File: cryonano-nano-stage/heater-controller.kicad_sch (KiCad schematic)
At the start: 0 parts

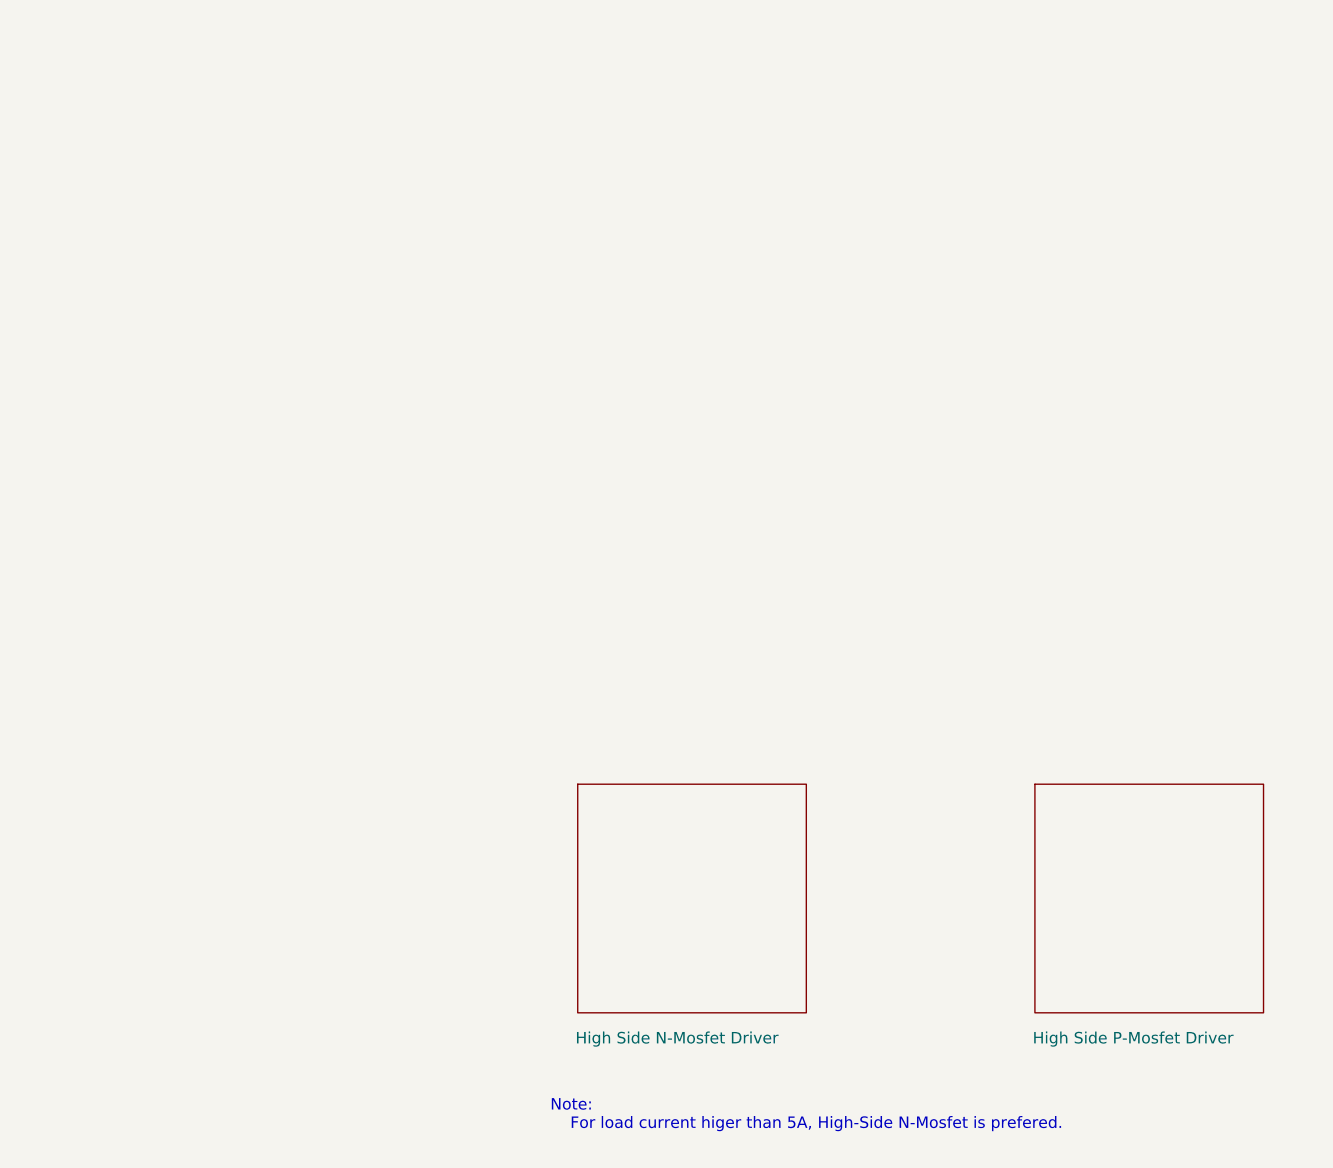
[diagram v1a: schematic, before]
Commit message: sch improved
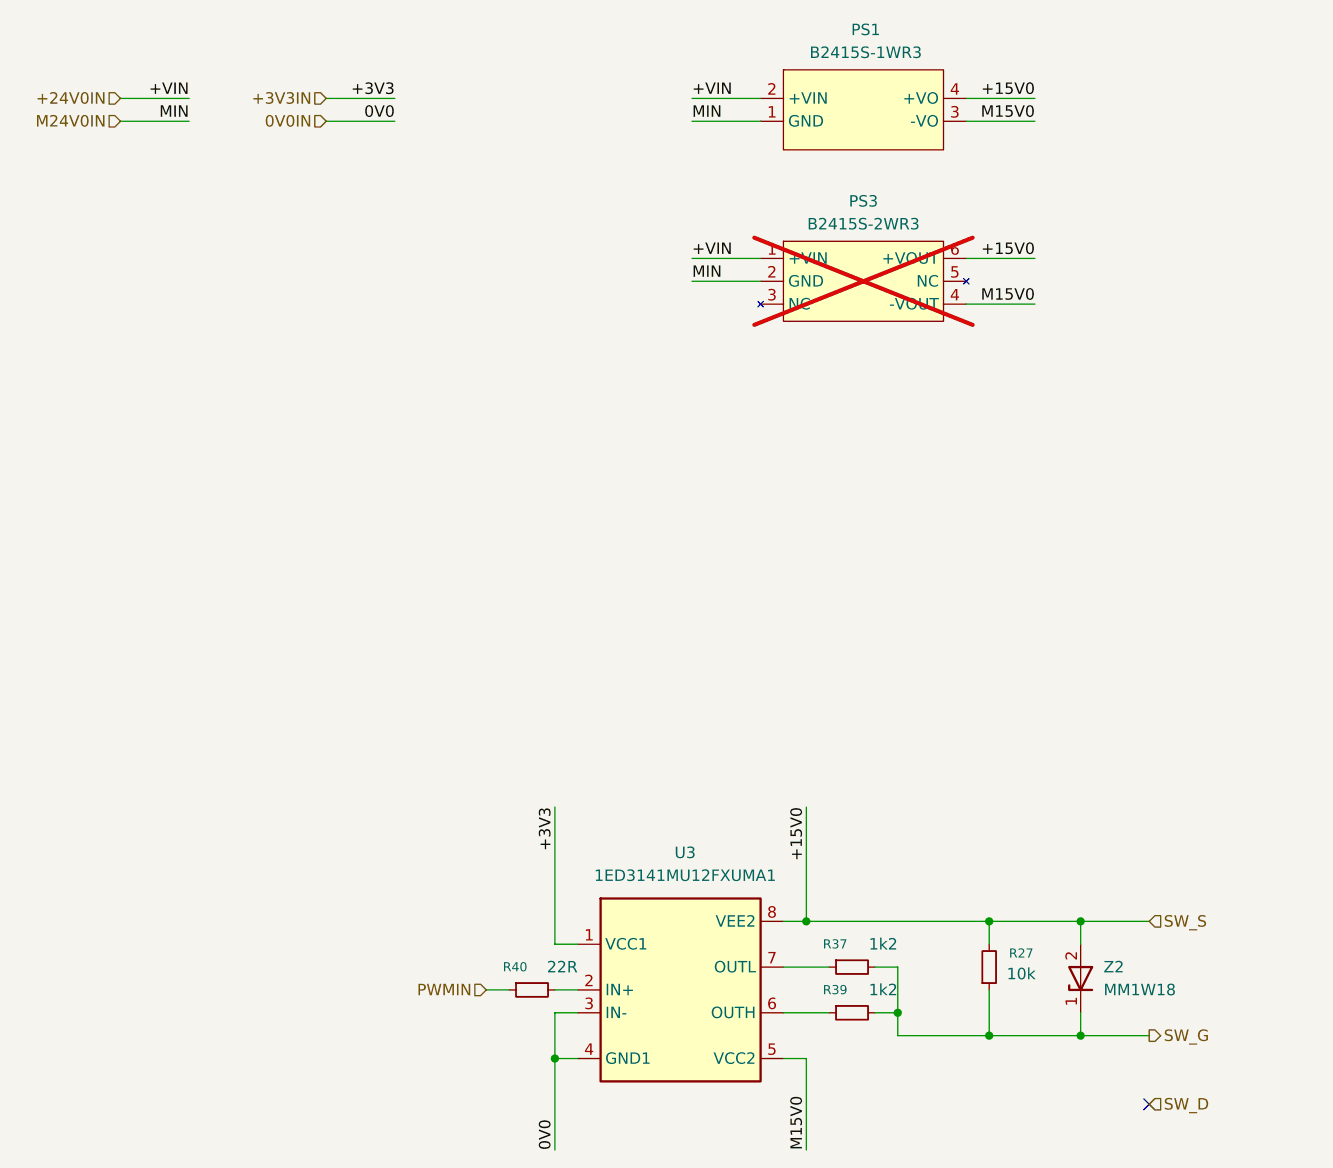
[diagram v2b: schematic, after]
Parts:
- added PS1: B2415S-1WR3, SamacSys_Parts:HLKB2405S2WR3, symbol symbols:BxxxxS-1WR3
- added PS3: B2415S-2WR3, symbol symbols:BxxxxS-2WR3
- added R27: 10k, Resistor_SMD:R_0603_1608Metric, symbol Device:R_Small
- added R37, R39: 1k2, Resistor_SMD:R_0603_1608Metric, symbol Device:R_Small
- added R40: 22R, Resistor_SMD:R_0603_1608Metric, symbol Device:R_Small
- added U3: 1ED3141MU12FXUMA1, SOIC127P600X175-8N, symbol symbols:1ED3141MU12FXUMA1
- added Z2: MM1W18, Diode_SMD:D_SOD-123, symbol symbols:MM1W18
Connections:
- new net: R39.1, U3.6 (OUTH)
- new net: R40.2, U3.2 (IN+)
- new net: R37.1, U3.7 (OUTL)
- new net +24V0IN: PS1.2 (+VIN), PS3.1 (+VIN)
- new net +3V3IN: U3.1 (VCC1)
- new net 0V0IN: U3.3 (IN-), U3.4 (GND1)
- new net M15V0: PS1.3 (-VO), PS3.4 (-VOUT), U3.5 (VCC2)
- new net M24V0IN: PS1.1 (GND), PS3.2 (GND)
- new net PWMIN: R40.1
- new net SW_G: R27.1, R37.2, R39.2, Z2.1 (C)
- new net SW_S: PS1.4 (+VO), PS3.6 (+VOUT), R27.2, U3.8 (VEE2), Z2.2 (A)
- no-connect marks 0 -> 1
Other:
- removed sheet High Side N-Mosfet Driver
- removed sheet High Side P-Mosfet Driver
- note removed: "Note: For load current higer than 5A, High-Side N-Mosfet is prefered."
- company: (none) -> Cryonano Labs Pvt. Ltd.
- title: (none) -> Nano stage controller
